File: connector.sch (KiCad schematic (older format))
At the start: 3 parts, among them J1 DB26_Male_HighDensity_Mountin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, J6 Conn_02x02_Odd_Even, SW3 SW_SPST

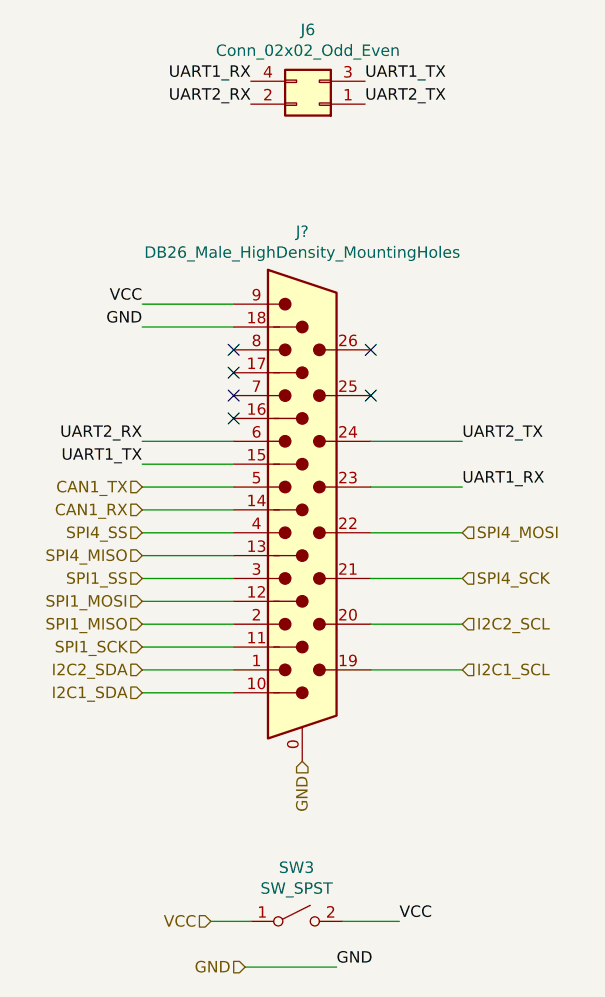
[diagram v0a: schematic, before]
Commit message: schematic improvements
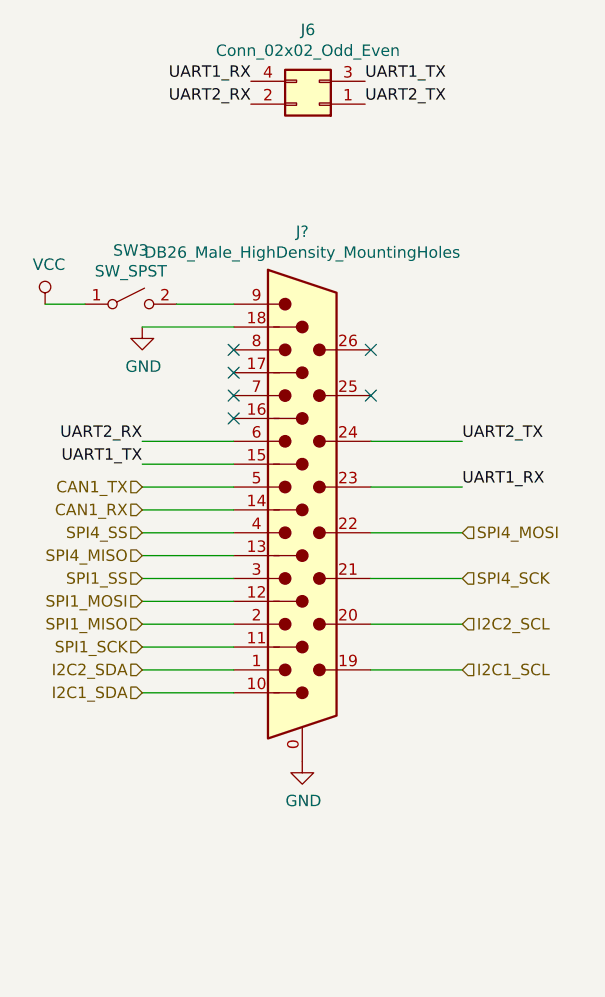
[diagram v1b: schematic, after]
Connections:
- net VCC: no longer J1.9, SW3.2 (B)
- new net: J1.9, SW3.2 (B)
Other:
- moved on the sheet: SW3
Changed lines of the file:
@@
 Text HLabel 4725 5000 0    50   Input ~ 0
 I2C1_SDA
-Text HLabel 5425 5300 3    50   Input ~ 0
-GND
 Text HLabel 6125 4900 2    50   Input ~ 0
 I2C1_SCL
@@
 Text HLabel 6125 4300 2    50   Input ~ 0
 SPI4_MOSI
-Text HLabel 5025 6000 0    50   Input ~ 0
-VCC
-Text HLabel 5175 6200 0    50   Input ~ 0
-GND
 Text HLabel 4725 4500 0    50   Input ~ 0
 SPI1_SS
@@
 L Switch:SW_SPST SW3
 U 1 1 5F134DBC
-P 5400 6000
+P 4675 3300
 AR Path="/5F06A0A3/5F134DBC" Ref="SW3"  Part="1"
 AR Path="/5F152747/5F134DBC" Ref="SW1"  Part="1"
@@
 AR Path="/5F1649A2/5F134DBC" Ref="SW?"  Part="1"
 AR Path="/5F1649C4/5F134DBC" Ref="SW?"  Part="1"
-F 0 "SW?" H 5400 6235 50  0000 C CNN
-F 1 "SW_SPST" H 5400 6144 50  0000 C CNN
-F 2 "" H 5400 6000 50  0001 C CNN
-F 3 "~" H 5400 6000 50  0001 C CNN
-	1    5400 6000
-	1    0    0    -1
-$EndComp
-Wire Wire Line
-	5200 6000 5025 6000
-Wire Wire Line
-	5600 6000 5850 6000
+F 0 "SW?" H 4675 3535 50  0000 C CNN
+F 1 "SW_SPST" H 4675 3444 50  0000 C CNN
+F 2 "" H 4675 3300 50  0001 C CNN
+F 3 "~" H 4675 3300 50  0001 C CNN
+	1    4675 3300
+	1    0    0    -1
+$EndComp
+Wire Wire Line
+	4475 3300 4300 3300
+Wire Wire Line
+	4875 3300 5125 3300
 $Comp
 L Connector_Generic:Conn_02x02_Odd_Even J6
@@
 UART2_TX
 Wire Wire Line
-	5575 6200 5175 6200
-Text Label 5575 6200 0    50   ~ 0
-GND
-Text Label 5850 6000 0    50   ~ 0
-VCC
-Text Label 4725 3300 2    50   ~ 0
-VCC
-Text Label 4725 3400 2    50   ~ 0
-GND
-Wire Wire Line
-	5125 3300 4725 3300
-Wire Wire Line
 	5125 3400 4725 3400
+$Comp
+L power:VCC #PWR?
+U 1 1 5F4B6D92
+P 4300 3300
+F 0 "#PWR?" H 4300 3150 50  0001 C CNN
+F 1 "VCC" H 4317 3473 50  0000 C CNN
+F 2 "" H 4300 3300 50  0001 C CNN
+F 3 "" H 4300 3300 50  0001 C CNN
+	1    4300 3300
+	1    0    0    -1
+$EndComp
+$Comp
+L power:GND #PWR?
+U 1 1 5F4B7169
+P 4725 3400
+F 0 "#PWR?" H 4725 3150 50  0001 C CNN
+F 1 "GND" H 4730 3227 50  0000 C CNN
+F 2 "" H 4725 3400 50  0001 C CNN
+F 3 "" H 4725 3400 50  0001 C CNN
+	1    4725 3400
+	1    0    0    -1
+$EndComp
+$Comp
+L power:GND #PWR?
+U 1 1 5F4B88F0
+P 5425 5300
+F 0 "#PWR?" H 5425 5050 50  0001 C CNN
+F 1 "GND" H 5430 5127 50  0000 C CNN
+F 2 "" H 5425 5300 50  0001 C CNN
+F 3 "" H 5425 5300 50  0001 C CNN
+	1    5425 5300
+	1    0    0    -1
+$EndComp
 $EndSCHEMATC
